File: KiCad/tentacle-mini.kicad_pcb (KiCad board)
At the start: 2 copper layers, 68.6 x 53.3 mm, 24 parts, among them P102 INT-DIS, P201 BNC, P202 BNC, P301 BNC, P302 CHANNEL 5, P303 CHANNEL 4, U201 whitebox-isolator, U202 whitebox-isolator

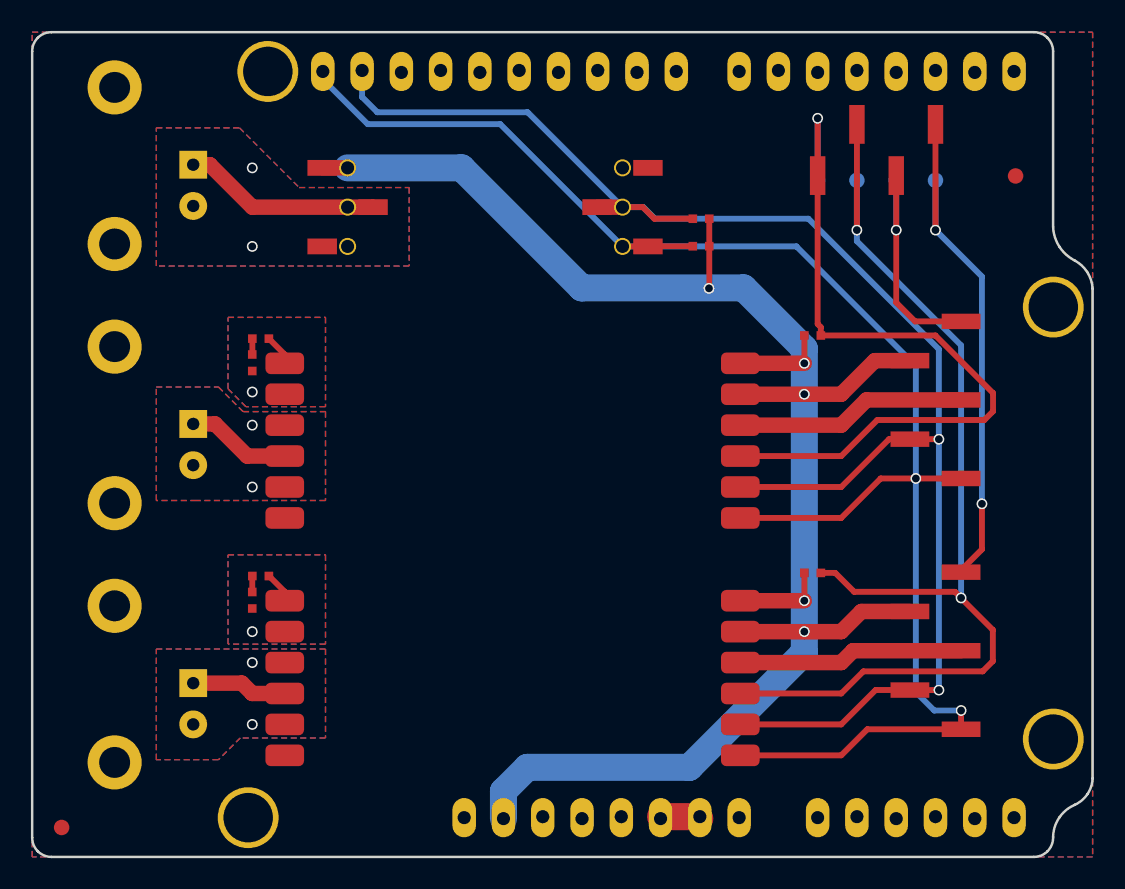
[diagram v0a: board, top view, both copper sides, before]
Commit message: update for SMA
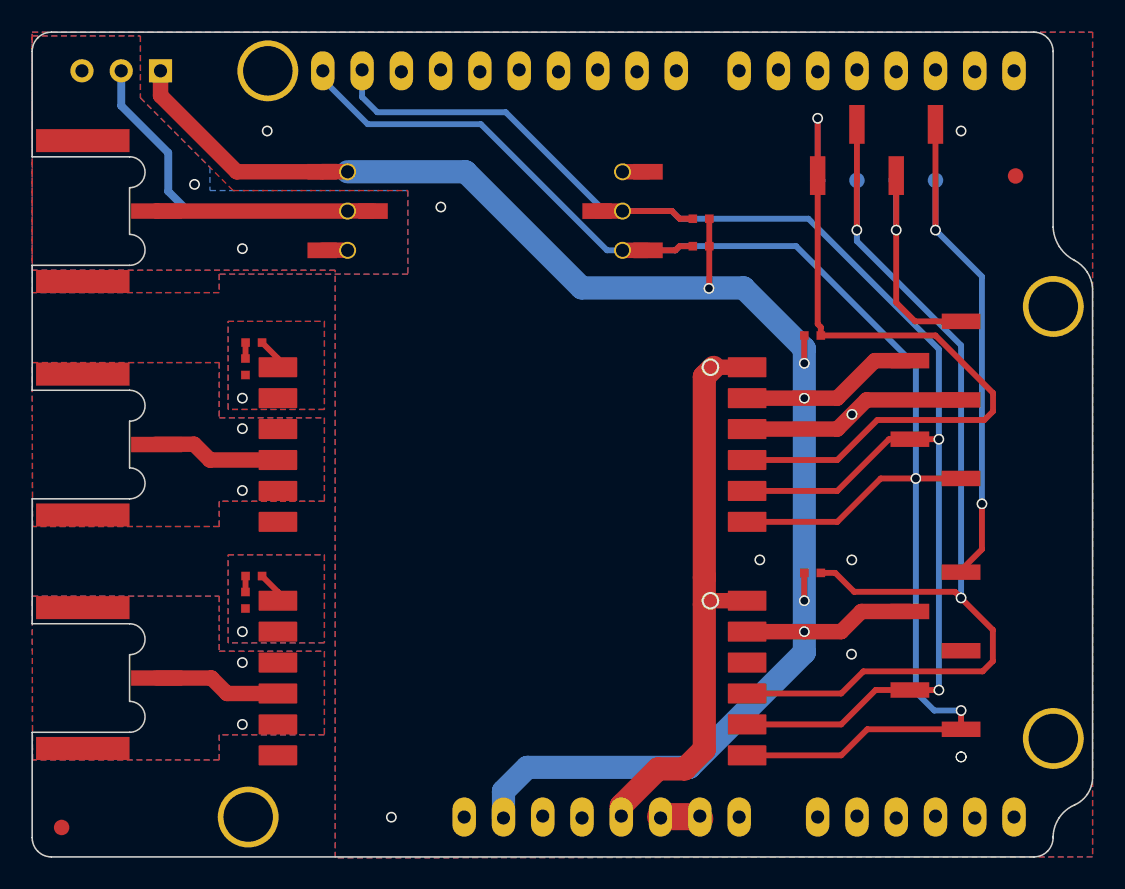
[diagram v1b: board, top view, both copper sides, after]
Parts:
- added J1: EZO_Flow, tentacle:WB-1x3-pin-header-handsolder, F.Cu at (135.3, 78.7)
- P201, P202, P301: value BNC -> SMA; footprint tentacle:WB-BNC -> tentacle:WB-SMA_EDGES_CORNER
- R101, R102: value 4.7K -> 4K7
- R201, R202: value R -> 220R
- U201, U202: value whitebox-isolator -> WHITEBOX T0; footprint tentacle:WB-T0-isolator -> tentacle:WB-T0-isolator-temporary-bugfix
- fiducial: value VAL** -> FIDUCIAL 1
- fiducial: value VAL** -> FIDUCIAL 2
- moved P301 6.09 mm to (127.0, 87.8)
- moved P202 5.48 mm to (127.0, 102.9)
- moved P201 5.35 mm to (127.0, 118.0)
- moved D202 0.51 mm to (140.8, 97.8)
- moved R202 0.51 mm to (141.3, 96.3)
- moved D201 0.44 mm to (140.8, 112.9)
- moved R201 0.44 mm to (141.3, 111.4)
- moved STP301 0.25 mm to (156.3, 87.8)
- moved U202 0.25 mm to (158.1, 102.9)
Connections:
- SHIELD101 pad 0: (no net) -> Net-(SHIELD101-Pad0)
- SHIELD101 pad 1: (no net) -> Net-(SHIELD101-Pad1)
- SHIELD101 pad 10: (no net) -> Net-(SHIELD101-Pad10)
- SHIELD101 pad 11: (no net) -> Net-(SHIELD101-Pad11)
- SHIELD101 pad 12: (no net) -> Net-(SHIELD101-Pad12)
- SHIELD101 pad 13: (no net) -> Net-(SHIELD101-Pad13)
- SHIELD101 pad 2: (no net) -> Net-(SHIELD101-Pad2)
- SHIELD101 pad 3: (no net) -> Net-(SHIELD101-Pad3)
- SHIELD101 pad 3V3: (no net) -> Net-(SHIELD101-Pad3V3)
- SHIELD101 pad 4: (no net) -> Net-(SHIELD101-Pad4)
- SHIELD101 pad 5: (no net) -> Net-(SHIELD101-Pad5)
- SHIELD101 pad 5V: (no net) -> 5V
- SHIELD101 pad 6: (no net) -> Net-(SHIELD101-Pad6)
- SHIELD101 pad 7: (no net) -> Net-(SHIELD101-Pad7)
- SHIELD101 pad 8: (no net) -> Net-(SHIELD101-Pad8)
- SHIELD101 pad 9: (no net) -> Net-(SHIELD101-Pad9)
- SHIELD101 pad AD0: (no net) -> Net-(SHIELD101-PadAD0)
- SHIELD101 pad AD1: (no net) -> Net-(SHIELD101-PadAD1)
- SHIELD101 pad AD2: (no net) -> Net-(SHIELD101-PadAD2)
- SHIELD101 pad AD3: (no net) -> Net-(SHIELD101-PadAD3)
- SHIELD101 pad AD4: (no net) -> Net-(SHIELD101-PadAD4)
- SHIELD101 pad AD5: (no net) -> Net-(SHIELD101-PadAD5)
- SHIELD101 pad AREF: (no net) -> Net-(SHIELD101-PadAREF)
- SHIELD101 pad NC: (no net) -> Net-(SHIELD101-PadNC)
- SHIELD101 pad RST: (no net) -> Net-(SHIELD101-PadRST)
- SHIELD101 pad V_IN: (no net) -> Net-(SHIELD101-PadV_IN)
- U201 pad 12: Vioref -> 5V
- U201 pad 6: (no net) -> Net-(U201-Pad6)
- U202 pad 12: Vioref -> 5V
- U202 pad 6: (no net) -> Net-(U202-Pad6)
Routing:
- net 5V: track 0.00 -> 37.7 mm
- net /nonisochannels/PRB3: track 12.8 -> 35.2 mm
- net GND: track 32.1 -> 18.9 mm, vias 0 -> 10
- net Vioref: track 120.4 -> 125.3 mm
- net /isochannels/PRB1: track 6.20 -> 8.26 mm
- net /nonisochannels/PRBGND3: track 0.00 -> 1.65 mm
- net /isochannels/PRB2: track 6.78 -> 8.32 mm
- net /SDA: track 102.1 -> 101.2 mm
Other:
- outline, holes or cut-outs redrawn
